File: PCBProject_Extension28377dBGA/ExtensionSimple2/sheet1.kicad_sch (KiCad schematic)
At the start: 88 parts, among them J1 Conn_02x08_Top_Bottom, J2 Conn_01x02_Pin, Q1 FMMT618TA, U1 SN74ABT541, U2 SN74ABT541

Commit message: extension board layout
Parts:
- removed INC2: HIF3FC-20PA-2.54DSA, Connector_IDC:IDC-Header_2x10_P2.54mm_Vertical, symbol sheet1-altium-import:root_0_HIF3FC-20PA-2.54DSA
- added J1: Conn_02x05_Odd_Even, Connector_IDC:IDC-Header_2x05_P2.54mm_Vertical, symbol Connector_Generic:Conn_02x05_Odd_Even
- LEM1, LEM2: footprint Connector_IDC:IDC-Header_2x15_P2.54mm_Vertical -> Connector_PinSocket_2.54mm:PinSocket_2x15_P2.54mm_Vertical
- RU3: footprint mmlab-footprint-library:0805 -> Resistor_SMD:R_0805_2012Metric
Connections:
- net AGND: now also J1.9 (Pin_9)
- net D+5V: now also J1.10 (Pin_10)
- net MQEP1A: now also J1.2 (Pin_2)
- net MQEP1B: now also J1.4 (Pin_4)
- net MQEP1Z: now also J1.6 (Pin_6)
- net PE_GND: now also J1.7 (Pin_7)
- net QEP1_HALL_U: now also J1.1 (Pin_1)
- net QEP1_HALL_V: now also J1.3 (Pin_3)
- net QEP1_HALL_W: now also J1.5 (Pin_5)
- net VDD: now also J1.8 (Pin_8)
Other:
- moved on the sheet: J1

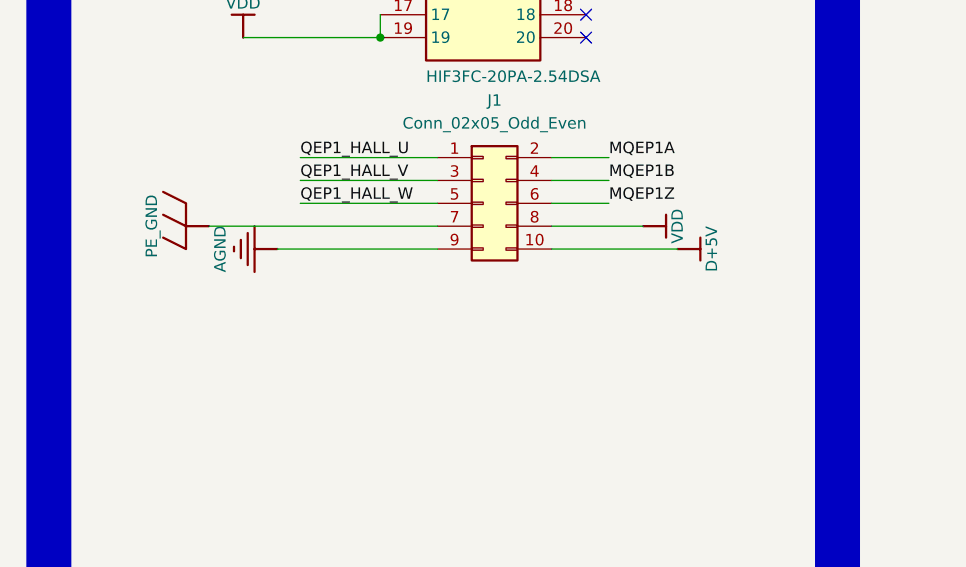
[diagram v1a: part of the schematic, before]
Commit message: HY加油
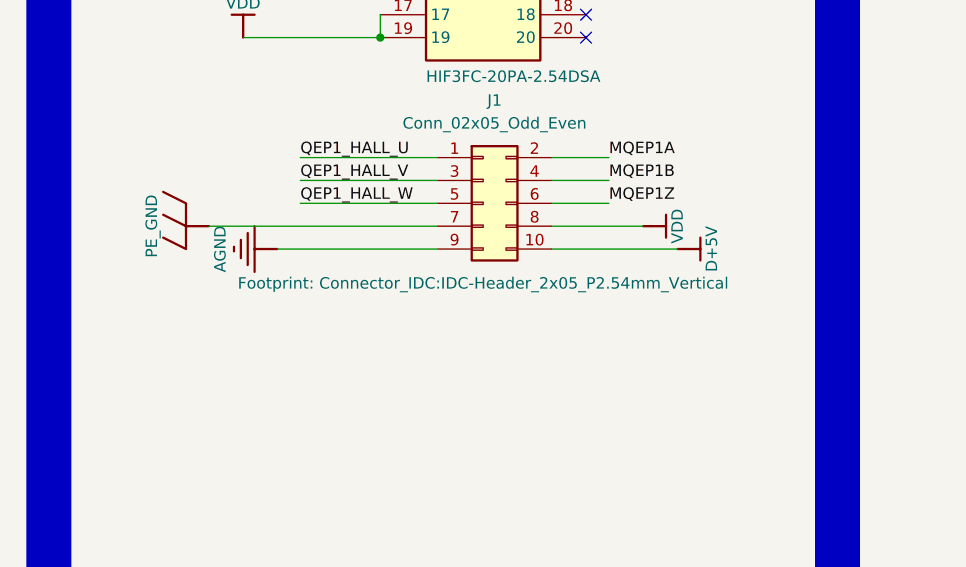
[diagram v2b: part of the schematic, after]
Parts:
- DSP1: footprint 1mmlab_footprint:DSP_240 -> 1mmlab_footprint:DSP_240_SMD
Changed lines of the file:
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@@
       (effects (font (size 1.27 1.27)))
     )
-    (property "Footprint" "1mmlab_footprint:DSP_240" (at 711.2 421.64 0)
+    (property "Footprint" "1mmlab_footprint:DSP_240_SMD" (at 711.2 421.64 0)
       (effects (font (size 1.27 1.27)) hide)
     )
@@
   )
   (symbol (lib_id "Connector_Generic:Conn_02x05_Odd_Even") (at 400.05 509.27 0) (unit 1)
-    (in_bom yes) (on_board yes) (dnp no) (fields_autoplaced)
+    (in_bom yes) (on_board yes) (dnp no)
     (property "Reference" "J1" (at 401.32 497.84 0)
       (effects (font (size 1.27 1.27)))
@@
       (effects (font (size 1.27 1.27)))
     )
-    (property "Footprint" "Connector_IDC:IDC-Header_2x05_P2.54mm_Vertical" (at 400.05 509.27 0)
-      (effects (font (size 1.27 1.27)) hide)
+    (property "Footprint" "Connector_IDC:IDC-Header_2x05_P2.54mm_Vertical" (at 400.05 518.16 0) (show_name)
+      (effects (font (size 1.27 1.27)))
     )
     (property "Datasheet" "~" (at 400.05 509.27 0)
